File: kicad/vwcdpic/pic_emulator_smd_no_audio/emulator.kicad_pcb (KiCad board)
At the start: 2 copper layers, 15.6 x 14.2 mm, 14 parts, among them U1 PIC12F629, U2 LM78L05ACZ

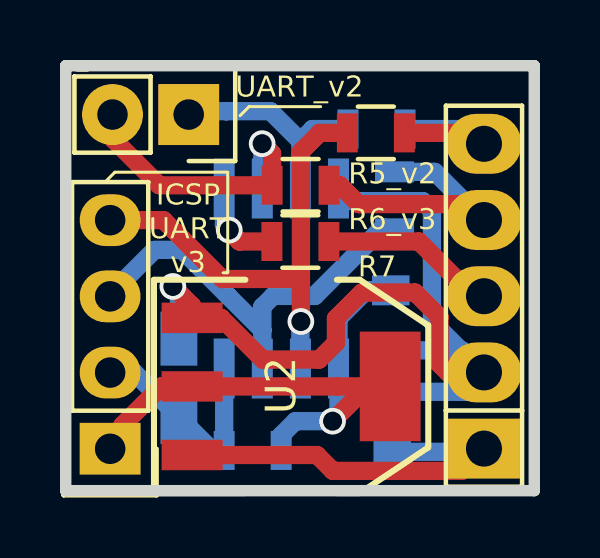
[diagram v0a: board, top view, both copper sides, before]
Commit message: revert to version 3 based
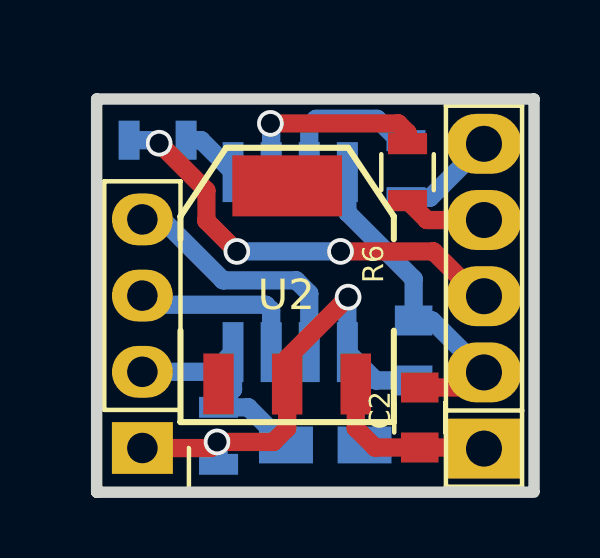
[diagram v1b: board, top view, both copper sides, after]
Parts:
- removed R5_v2, R6_v2: 3k3, Resistors_SMD:R_0805
- removed UART_v2: CONN_01X04, Pin_Headers:Pin_Header_Straight_1x02
- C2: moved to F.Cu
- R7: moved to B.Cu
- moved R7 5.83 mm to (139.8, 115.7), turned to 180 degrees
- moved C1 5.36 mm to (145.4, 125.9), turned to 0 degrees
- moved R6 3.59 mm to (148.1, 116.8), turned to 270 degrees
- moved U2 3.39 mm to (144.1, 120.5), turned to 0 degrees
- moved R5 1.66 mm to (148.1, 116.7), turned to 270 degrees
- moved C10 1.26 mm to (148.3, 122.7), turned to 90 degrees
- moved R1 1.24 mm to (141.8, 125.6), turned to 270 degrees
- moved ICSP_UART1 1.07 mm to (139.3, 126.0)
- moved C2 0.93 mm to (148.5, 125.0)
- moved U1 0.62 mm to (144.2, 119.8)
- renumbered ICSP to ICSP_UART1, R5_v3 to R5, R6_v3 to R6
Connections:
- net /MCLR_VPP renamed Net-(C1-Pad1)
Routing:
- net GND: track 33.2 -> 11.3 mm, vias 1 -> 0
- net Net-(ICSP_UART1-Pad3): track 17.7 -> 5.89 mm
- net DataOut: track 6.09 -> 15.0 mm, vias 0 -> 3
- net Net-(ICSP_UART1-Pad4): track 16.3 -> 8.54 mm, vias 1 -> 0
- net POWER_CTL: track 13.4 -> 6.18 mm
- net DataIn: track 9.29 -> 2.85 mm
- net +5V: track 20.6 -> 15.5 mm, vias 1 -> 2
- net Net-(R6-Pad1): track 9.78 -> 6.70 mm
- net Net-(R5-Pad1): track 7.53 -> 5.17 mm
- net CLK: track 5.13 -> 3.34 mm
- net Net-(R7-Pad1): track 3.20 -> 2.01 mm, vias 1 -> 0
- added copper zone on B.Cu, net GND
- added copper zone on F.Cu, net GND
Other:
- board size 15.6 x 14.2 mm -> 14.6 x 13.1 mm
- board text removed: "ICSP UART v3"

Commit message: cleanup
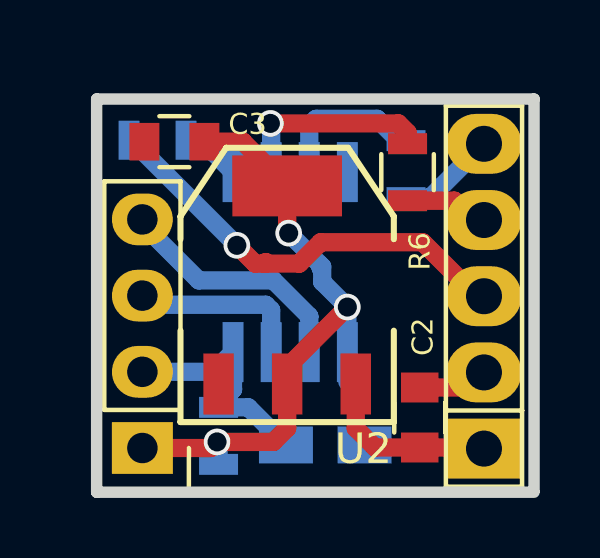
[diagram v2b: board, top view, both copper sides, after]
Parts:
- C3: renamed from C10; moved to F.Cu
- moved C3 10.6 mm to (140.4, 115.8), turned to 180 degrees
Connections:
- net CLK renamed CLK-PRG_DATA
- net DataIn renamed DataIn-PRG_CLK
- net Net-(C1-Pad1) renamed RESET
- net Net-(ICSP_UART1-Pad3) renamed PJRC
- net Net-(ICSP_UART1-Pad4) renamed ARCHOS
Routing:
- net GND: track 11.3 -> 2.40 mm
- net +5V: track 15.5 -> 21.9 mm, vias 2 -> 3
- net DataOut: track 15.0 -> 15.4 mm, vias 3 -> 1
